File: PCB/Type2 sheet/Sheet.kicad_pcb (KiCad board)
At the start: 2 copper layers, 139.7 x 49 mm, 46 parts, among them P1 C_0201_0603Metric_Pad0.64x0.4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, U1 MCP9700Ax-ELT, U10 ADS7830, U11 ADS7830, U2 MCP2562-E-MF, U3 ATtiny1616-M, U5 CD74HC4067SM, U6 MCP2515-xST, U7 DRV5055A1xDBZxQ1, U8 DRV5055A1xDBZxQ1, U9 ADS7830

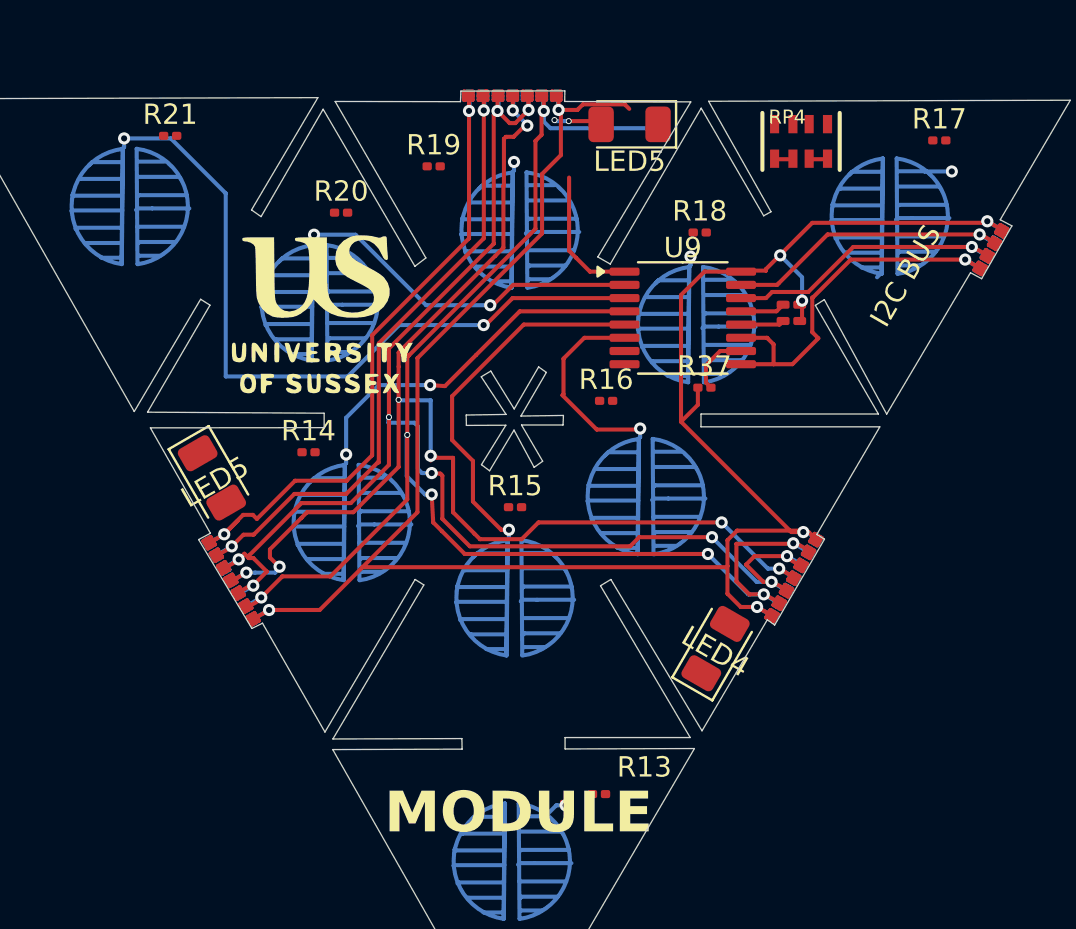
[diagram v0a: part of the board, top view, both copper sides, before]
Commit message: updates
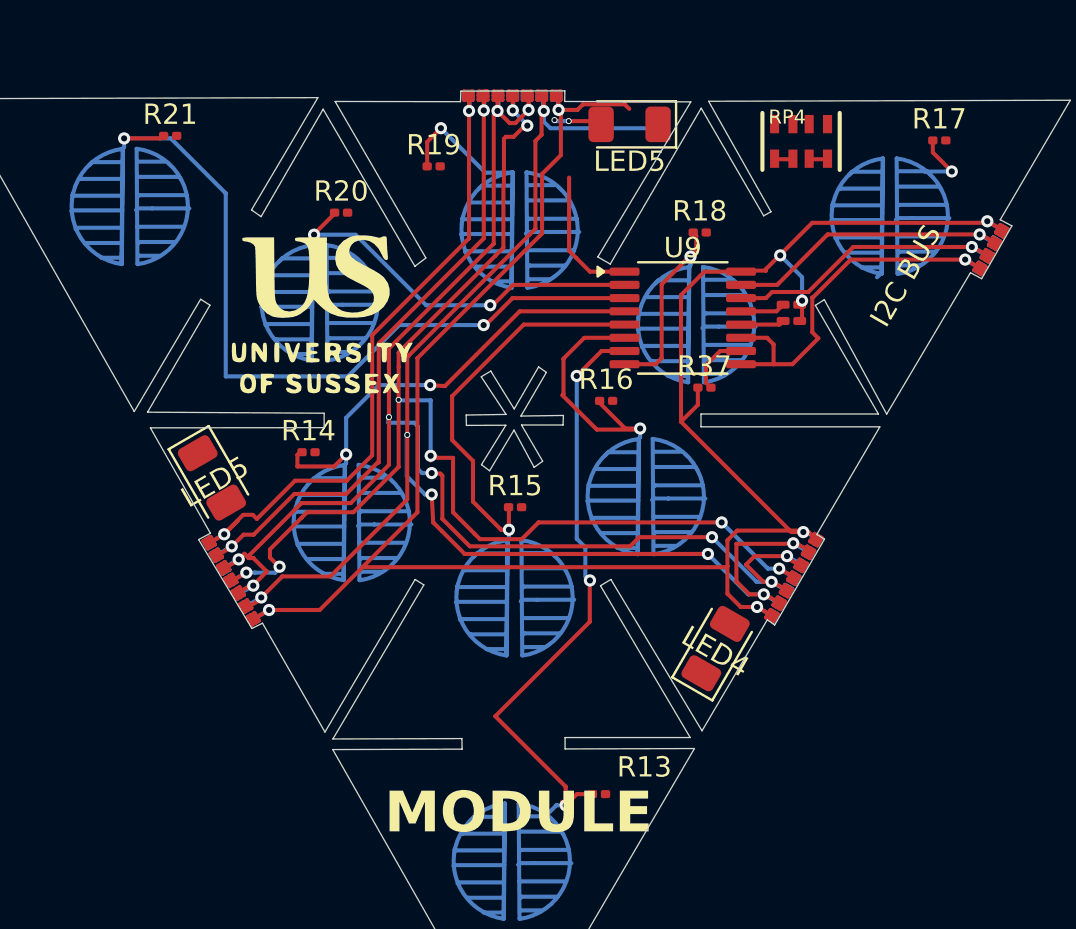
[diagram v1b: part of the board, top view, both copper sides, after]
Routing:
- net Net-(MK1--): track 18.8 -> 63.6 mm, vias 1 -> 7
- net Net-(U9-CH7): track 0.00 -> 7.52 mm
- net (no net): track 1747.8 -> 1740.6 mm, vias 128 -> 124
- net Net-(U9-CH3): track 18.4 -> 21.7 mm
- net Net-(U9-CH5): track 10.4 -> 13.0 mm
- net Net-(U9-CH2): track 37.2 -> 39.1 mm
- net Net-(U9-CH1): track 18.0 -> 19.5 mm
- net Net-(U9-CH4): track 18.6 -> 19.7 mm

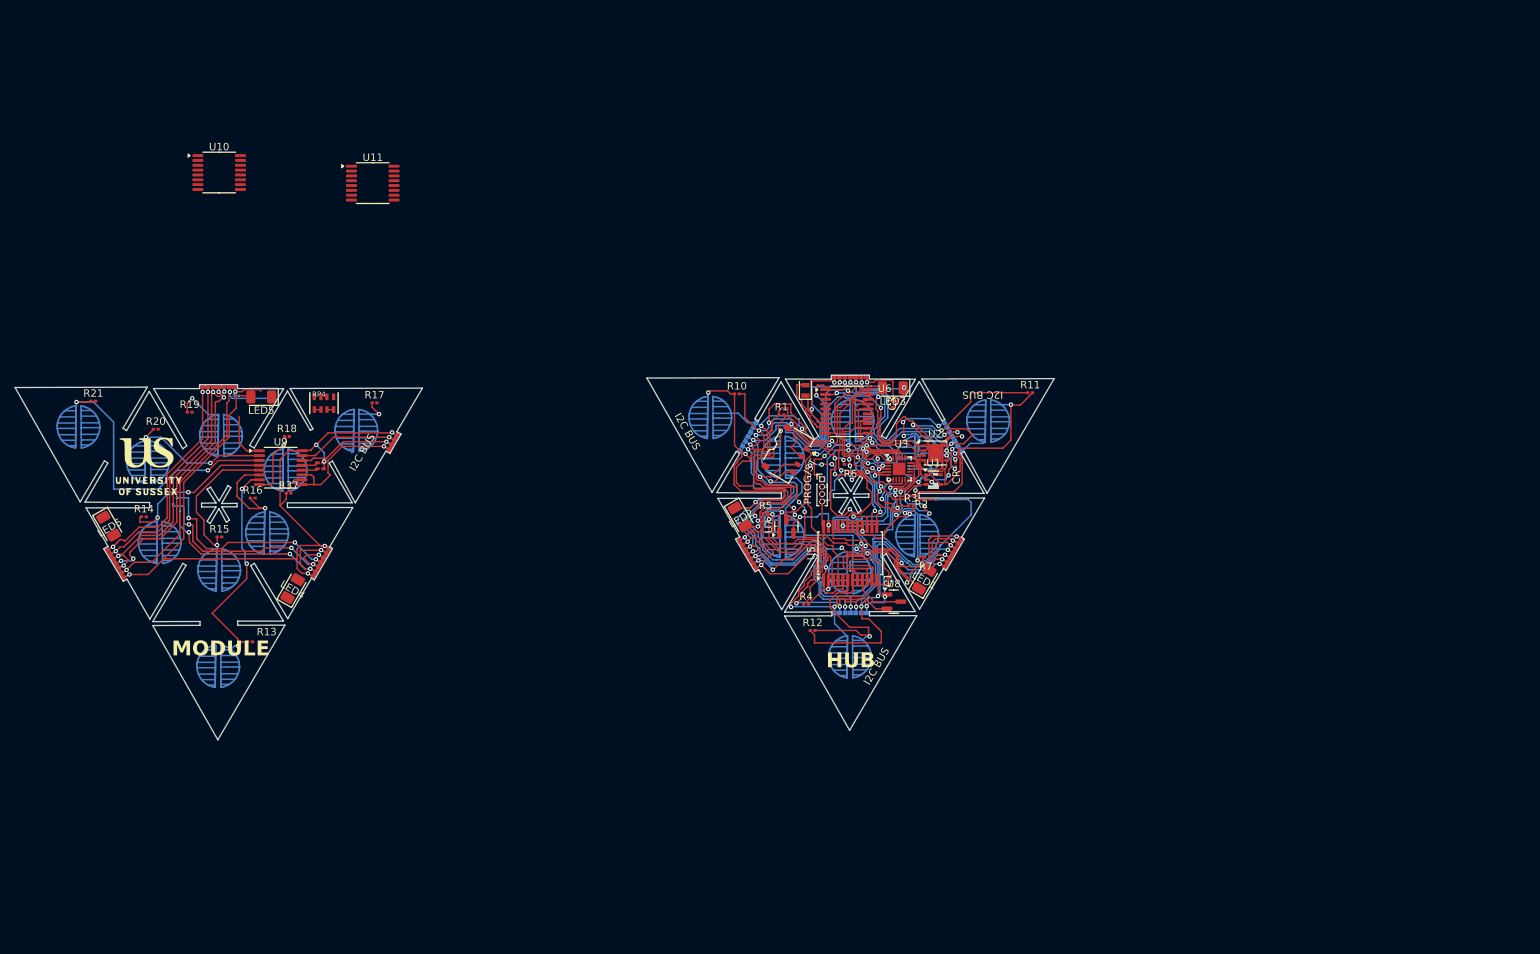
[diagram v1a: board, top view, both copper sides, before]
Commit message: new
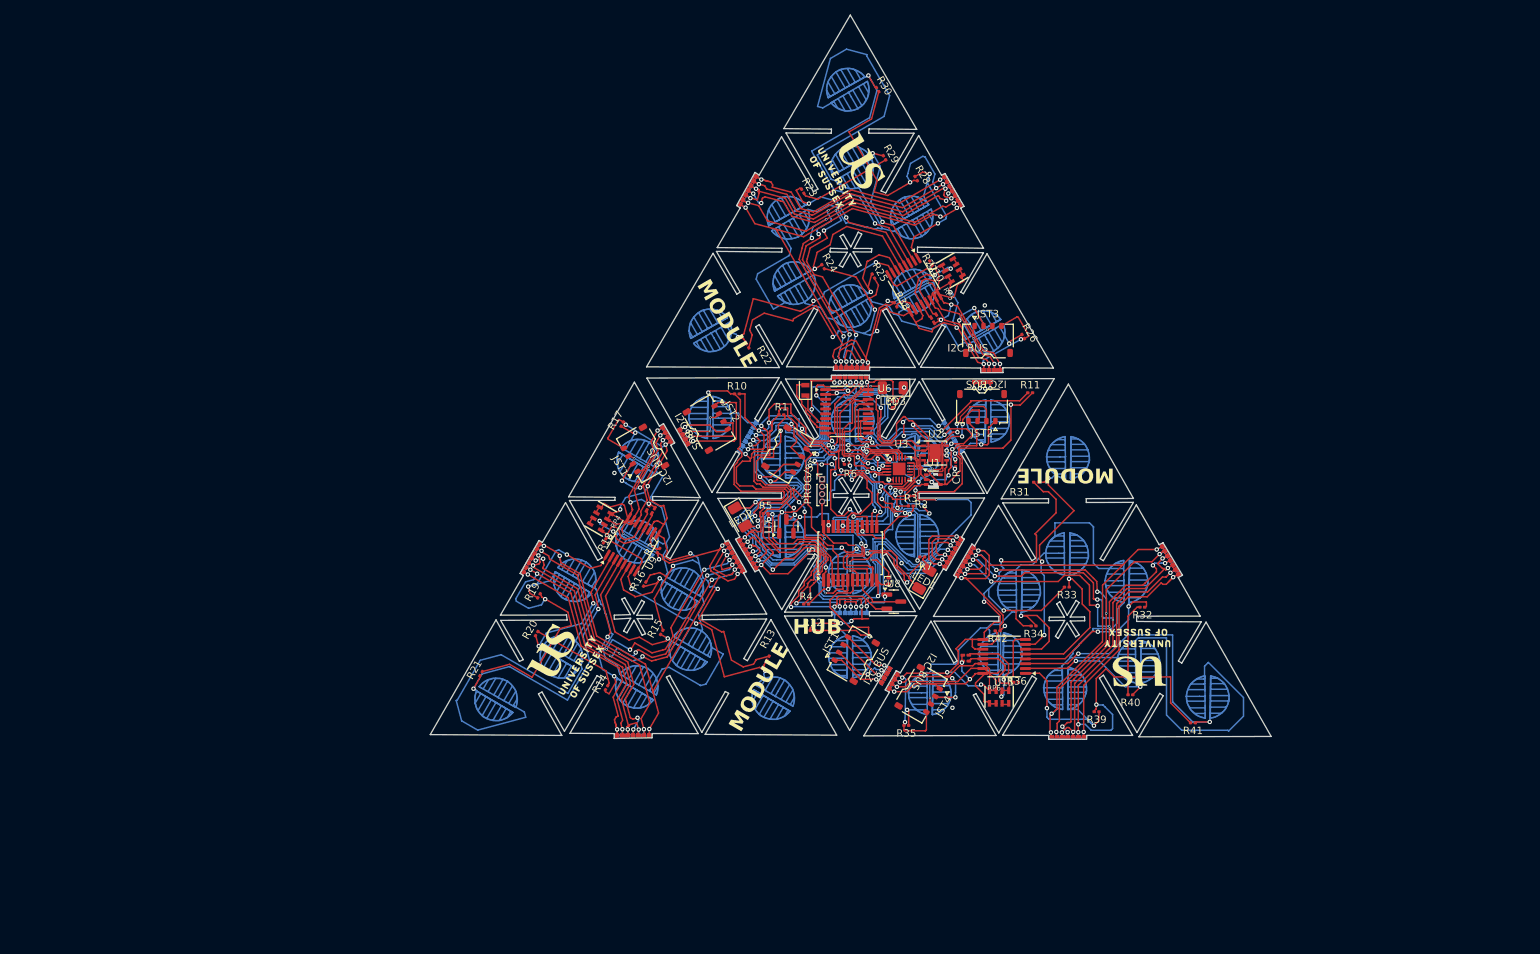
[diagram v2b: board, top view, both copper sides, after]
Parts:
- removed LED4, LED5 (x2): LED_1206_3216Metric, LED_SMD:LED_1206_3216Metric
- added G***1: LOGO, LOGO, F.Cu at (170.8, 47.5)
- added G***2: LOGO, LOGO, F.Cu at (209.7, 113.2)
- added JST1: JST_ACH_BM04B-ACHSS-A-GAN-ETF_1x04-1MP_P1.20mm_Vertical, Connector_JST:JST_ACH_BM04B-ACHSS-A-GAN-ETF_1x04-1MP_P1.20mm_Vertical, F.Cu at (143.1, 85.6)
- added JST1: JST_ACH_BM04B-ACHSS-A-GAN-ETF_1x04-1MP_P1.20mm_Vertical, Connector_JST:JST_ACH_BM04B-ACHSS-A-GAN-ETF_1x04-1MP_P1.20mm_Vertical, F.Cu at (171.4, 112.9)
- added JST2: JST_ACH_BM04B-ACHSS-A-GAN-ETF_1x04-1MP_P1.20mm_Vertical, Connector_JST:JST_ACH_BM04B-ACHSS-A-GAN-ETF_1x04-1MP_P1.20mm_Vertical, F.Cu at (188.7, 79.5)
- added JST2: JST_ACH_BM04B-ACHSS-A-GAN-ETF_1x04-1MP_P1.20mm_Vertical, Connector_JST:JST_ACH_BM04B-ACHSS-A-GAN-ETF_1x04-1MP_P1.20mm_Vertical, F.Cu at (152.0, 81.8)
- added JST3: JST_ACH_BM04B-ACHSS-A-GAN-ETF_1x04-1MP_P1.20mm_Vertical, Connector_JST:JST_ACH_BM04B-ACHSS-A-GAN-ETF_1x04-1MP_P1.20mm_Vertical, F.Cu at (189.5, 70.4)
- added JST4: JST_ACH_BM04B-ACHSS-A-GAN-ETF_1x04-1MP_P1.20mm_Vertical, Connector_JST:JST_ACH_BM04B-ACHSS-A-GAN-ETF_1x04-1MP_P1.20mm_Vertical, F.Cu at (180.5, 117.9)
- added P2: C_0201_0603Metric_Pad0.64x0.40mm_HandSolder, Capacitor_SMD:C_0201_0603Metric_Pad0.64x0.40mm_HandSolder, F.Cu at (182.1, 67.8)
- added P3: C_0201_0603Metric_Pad0.64x0.40mm_HandSolder, Capacitor_SMD:C_0201_0603Metric_Pad0.64x0.40mm_HandSolder, F.Cu at (182.8, 67.4)
- added P4: C_0201_0603Metric_Pad0.64x0.40mm_HandSolder, Capacitor_SMD:C_0201_0603Metric_Pad0.64x0.40mm_HandSolder, F.Cu at (186.5, 112.8)
- added P5: C_0201_0603Metric_Pad0.64x0.40mm_HandSolder, Capacitor_SMD:C_0201_0603Metric_Pad0.64x0.40mm_HandSolder, F.Cu at (186.5, 113.6)
- added R22: R, Resistor_SMD:R_0201_0603Metric, F.Cu at (157.2, 71.2)
- added R23: R, Resistor_SMD:R_0201_0603Metric, F.Cu at (164.6, 50.5)
- added R24: R, Resistor_SMD:R_0201_0603Metric, F.Cu at (167.3, 60.6)
- added R25: R, Resistor_SMD:R_0201_0603Metric, F.Cu at (174.1, 61.9)
- added R26: R, Resistor_SMD:R_0201_0603Metric, F.Cu at (194.2, 70.0)
- added R27: R, Resistor_SMD:R_0201_0603Metric, F.Cu at (181.8, 60.1)
- added R28: R, Resistor_SMD:R_0201_0603Metric, F.Cu at (179.9, 48.8)
- added R29: R, Resistor_SMD:R_0201_0603Metric, F.Cu at (175.6, 46.0)
- added R30: R, Resistor_SMD:R_0201_0603Metric, F.Cu at (174.7, 36.8)
- added R31: R, Resistor_SMD:R_0201_0603Metric, F.Cu at (196.0, 89.6)
- added R32: R, Resistor_SMD:R_0201_0603Metric, F.Cu at (210.3, 106.4)
- added R33: R, Resistor_SMD:R_0201_0603Metric, F.Cu at (200.1, 103.7)
- added R34: R, Resistor_SMD:R_0201_0603Metric, F.Cu at (195.6, 108.9)
- added R35: R, Resistor_SMD:R_0201_0603Metric, F.Cu at (178.5, 122.3)
- added R36: R, Resistor_SMD:R_0201_0603Metric, F.Cu at (193.3, 116.5)
- added R38: R, Resistor_SMD:R_0201_0603Metric, F.Cu at (177.1, 65.7)
- added R39: R, Resistor_SMD:R_0201_0603Metric, F.Cu at (204.1, 120.4)
- added R40: R, Resistor_SMD:R_0201_0603Metric, F.Cu at (208.7, 118.2)
- added R41: R, Resistor_SMD:R_0201_0603Metric, F.Cu at (217.1, 121.9)
- added R42: R, Resistor_SMD:R_0201_0603Metric, F.Cu at (190.8, 109.5)
- added RP5: 10K Pack, RESPACK_4X0603, F.Cu at (184.7, 61.1)
- added RP6: 10K Pack, RESPACK_4X0603, F.Cu at (191.0, 118.4)
- moved U11 106.1 mm to (191.7, 113.0), turned to 180 degrees
- moved U10 94.6 mm to (179.6, 63.1), turned to -60 degrees
- moved R13 69.6 mm to (159.9, 113.2), turned to 60 degrees
- moved R14 66.3 mm to (138.2, 117.2), turned to 60 degrees
- moved R21 63.7 mm to (121.4, 115.3), turned to 60 degrees
- moved G*** 61.7 mm to (132.6, 113.3), turned to 60 degrees
- moved R15 60.8 mm to (145.7, 109.8), turned to 60 degrees
- moved R20 58.1 mm to (128.8, 109.9), turned to 60 degrees
- moved R16 54.0 mm to (143.4, 103.3), turned to 60 degrees
- moved R19 53.0 mm to (129.1, 104.8), turned to 60 degrees
- moved R37 50.3 mm to (145.2, 98.8), turned to 60 degrees
- moved U9 48.4 mm to (141.7, 98.0), turned to 60 degrees
- moved P1 45.1 mm to (144.5, 93.4), turned to 60 degrees
- moved R18 45.0 mm to (138.0, 97.5), turned to 60 degrees
- moved P1 44.5 mm to (143.8, 93.0), turned to 60 degrees
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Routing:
- net (no net): track 1740.6 -> 3075.1 mm, vias 124 -> 190
- net Net-(MK1--): track 63.6 -> 491.8 mm, vias 7 -> 47
- net Net-(U1-V_{DD}): track 162.7 -> 456.8 mm, vias 16 -> 54
- net Net-(U9-CH0): track 6.75 -> 136.0 mm, vias 0 -> 7
- net Net-(U10-SDA): track 25.6 -> 102.3 mm, vias 3 -> 11
- net Net-(U10-CH0): track 0.00 -> 75.5 mm, vias 0 -> 3
- net Net-(U10-SCL): track 15.2 -> 86.5 mm, vias 2 -> 11
- net unconnected-(R20-Pad1): track 0.00 -> 39.0 mm, vias 0 -> 4
- net Net-(U9-CH1): track 19.5 -> 51.0 mm
- net Net-(U9-CH5): track 13.0 -> 32.7 mm, vias 1 -> 4
- net Net-(U9-CH4): track 19.7 -> 38.3 mm
- net Net-(U4-XOUT): track 14.4 -> 0.14 mm
- net unconnected-(U10-A0-Pad12): track 0.00 -> 12.0 mm, vias 0 -> 2
- net unconnected-(U11-A0-Pad12): track 0.00 -> 12.0 mm, vias 0 -> 2
- net unconnected-(U11-A1-Pad13): track 0.00 -> 10.4 mm
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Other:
- board size 139.7 x 49 mm -> 113 x 97.3 mm

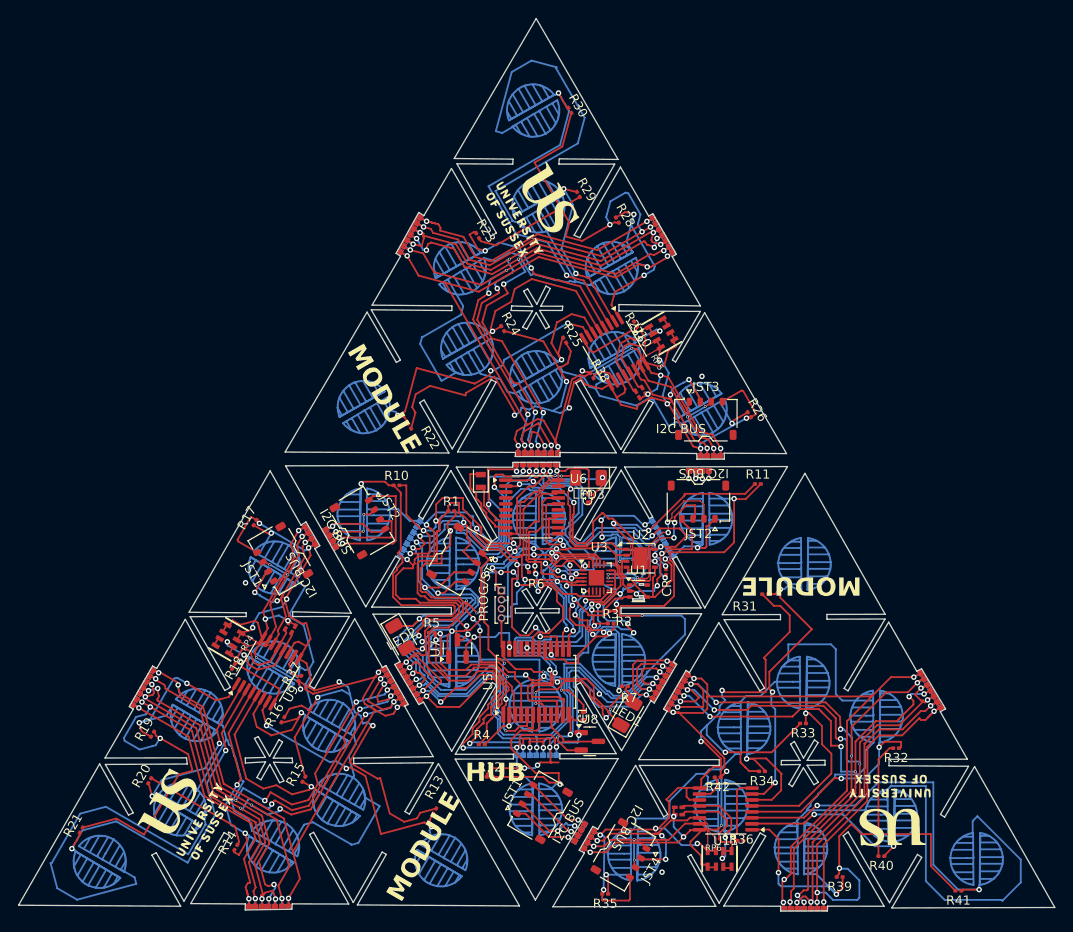
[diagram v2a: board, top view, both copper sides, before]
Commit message: Update Sheet.kicad_pcb
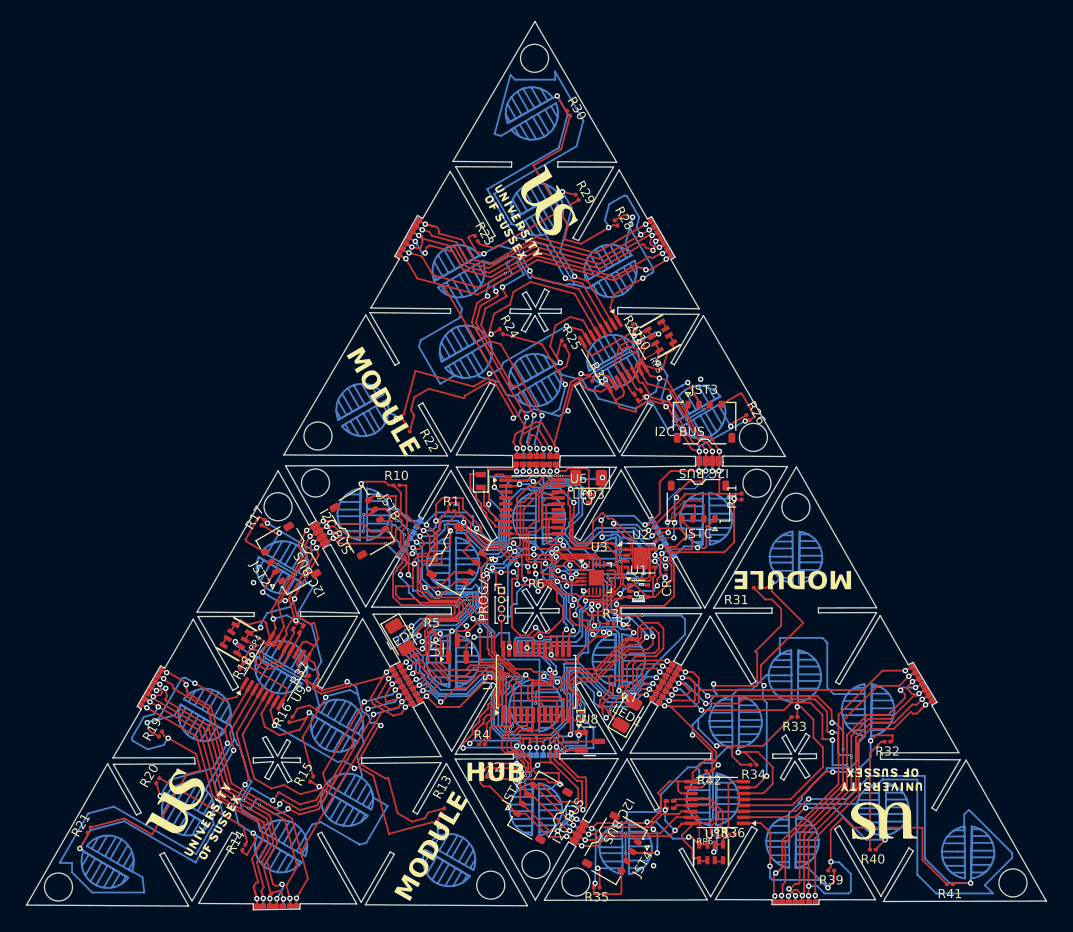
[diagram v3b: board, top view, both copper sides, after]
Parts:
- moved R11 2.23 mm to (193.4, 78.9), turned to 90 degrees
- moved R34 1.16 mm to (194.7, 108.2)
- moved R40 1.16 mm to (207.7, 117.4)
- moved JST4 1.16 mm to (179.6, 117.2)
- moved P4 1.16 mm to (185.6, 112.1)
- moved P5 1.16 mm to (185.6, 112.9)
- moved R32 1.16 mm to (209.3, 105.7)
- moved R36 1.16 mm to (192.4, 115.8)
- moved R41 1.16 mm to (216.1, 121.2)
- moved R42 1.16 mm to (189.9, 108.8)
- moved RP6 1.16 mm to (190.1, 117.7)
- moved U11 1.16 mm to (190.7, 112.3)
- moved G***2 1.16 mm to (208.8, 112.5)
- moved R31 1.16 mm to (195.1, 88.9)
- moved R33 1.16 mm to (199.2, 103.0)
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- renumbered JST1 to JST2, JST1 to JSTA, JST2 to JSTB, JST2 to JSTC
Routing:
- net Net-(U10-SCL): track 86.5 -> 196.9 mm, vias 11 -> 25
- net Net-(U5-I1): track 0.00 -> 84.5 mm, vias 0 -> 7
- net Net-(U5-I7): track 17.7 -> 74.2 mm, vias 1 -> 14
- net Net-(U5-I5): track 34.3 -> 88.6 mm, vias 3 -> 9
- net (no net): track 3075.1 -> 3022.7 mm, vias 190 -> 182
- net Net-(U1-V_{DD}): track 456.8 -> 472.8 mm, vias 54 -> 56
- net Net-(U10-SDA): track 102.3 -> 113.3 mm, vias 11 -> 10
- net Net-(MK1--): track 491.8 -> 495.7 mm
- net Net-(U2-CANH): track 162.8 -> 163.8 mm
- net Net-(U3-PB5): track 31.8 -> 31.3 mm
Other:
- board size 113 x 97.3 mm -> 111.2 x 96.9 mm
